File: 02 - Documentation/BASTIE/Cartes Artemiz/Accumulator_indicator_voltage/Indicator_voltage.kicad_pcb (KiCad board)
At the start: 2 copper layers, 82.4 x 42.6 mm, 22 parts, among them J7 2P Droit 2-11-2022, Q1 NMOS SQ2348ES-T1_GE3

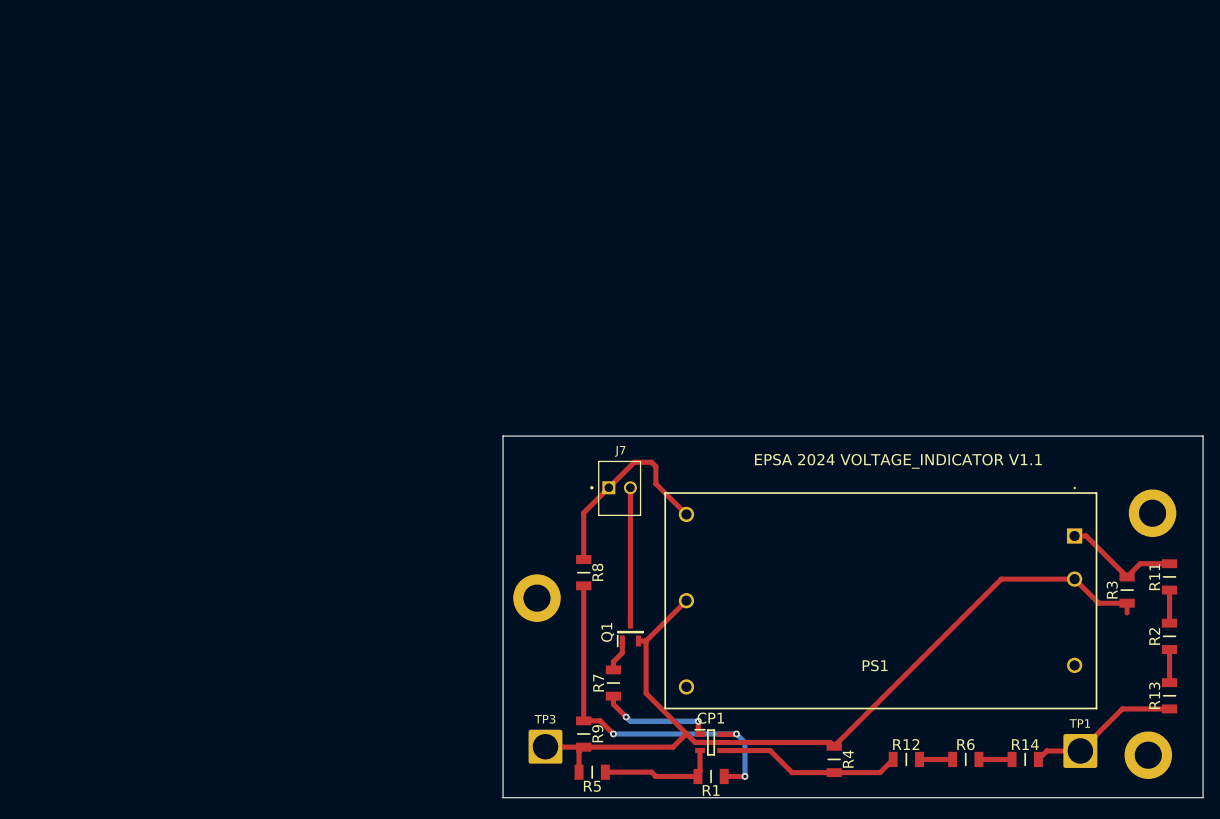
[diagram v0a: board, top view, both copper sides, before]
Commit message: Routage Voltage Indicator
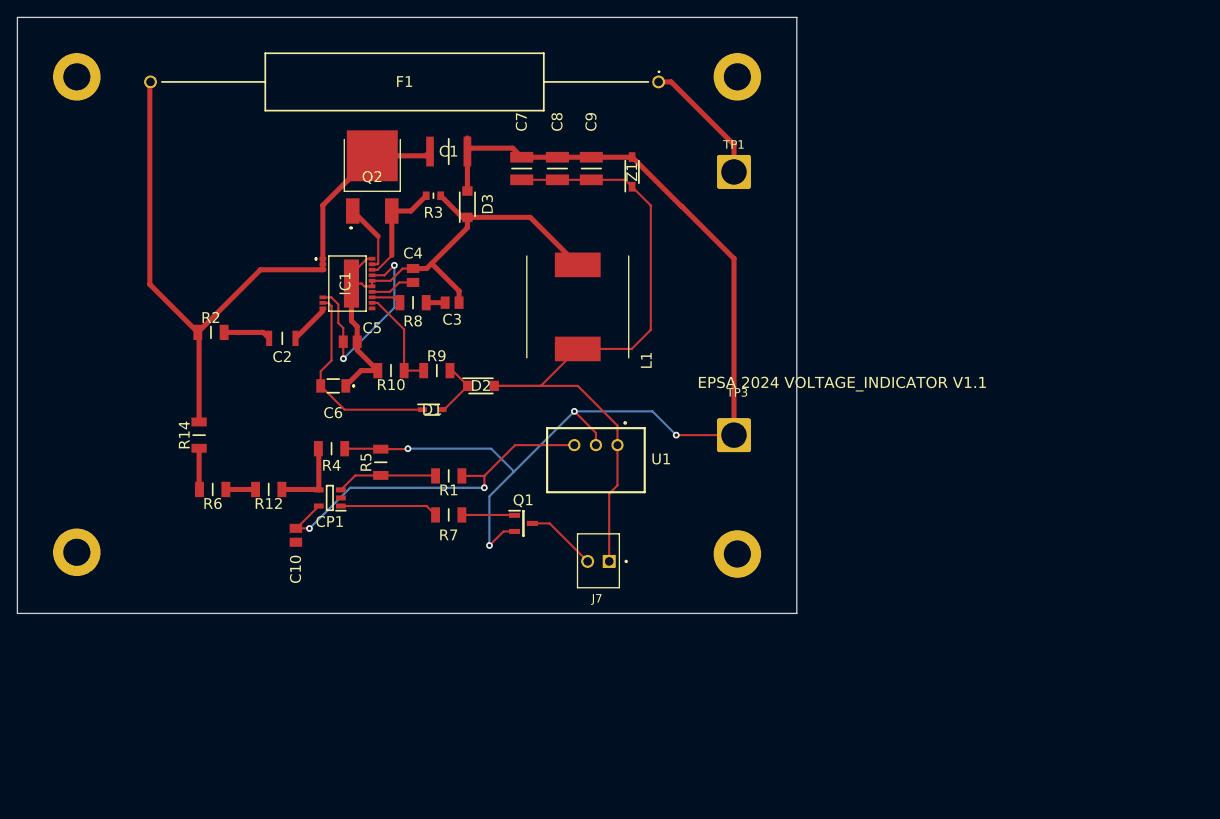
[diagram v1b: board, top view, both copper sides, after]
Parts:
- removed the ? at (93.0, 107.0)
- removed the ? at (165.5, 97.0)
- removed the ? at (165.0, 125.5)
- removed PS1: Alim HP EC7BW18-72S12, EPSA_lib:EC7BW1872S12
- removed R11, R13: 390k, EPSA_lib:RESC3216X70N
- added ?: , , F.Cu at (38.8, 101.6)
- added ?: , , F.Cu at (116.6, 45.6)
- added ?: , , F.Cu at (38.8, 45.6)
- added ?: , , F.Cu at (116.6, 101.8)
- added C1: 0.1u 630V, EPSA_lib:CAPC4532X200N, F.Cu at (82.6, 54.4)
- added C10: 10u, EPSA_lib:CAPC2012X130N, F.Cu at (64.6, 99.6)
- added C2: 10p 630V, EPSA_lib:CAPC3216X100N, F.Cu at (63.0, 76.4)
- added C3: 0.1u, EPSA_lib:CAPC2012X130N, F.Cu at (83.0, 72.2)
- added C4: 0.1u, EPSA_lib:CAPC2012X130N, F.Cu at (78.4, 69.0)
- added C5: 10u, EPSA_lib:CAPC2012X130N, F.Cu at (71.0, 76.8)
- added C6: 10u, EPSA_lib:GRM31x, F.Cu at (69.0, 82.0)
- added C7: 47u, EPSA_lib:CAPC3225X270N, F.Cu at (91.2, 56.4)
- added C8: 47u, EPSA_lib:CAPC3225X270N, F.Cu at (95.4, 56.4)
- added C9: 47u, EPSA_lib:CAPC3225X270N, F.Cu at (99.4, 56.4)
- added D1: Diode CMDSH2-3_TR_PBFREE, EPSA_lib:SOD2512X110N, F.Cu at (80.7, 84.8)
- added D2: Diode US1KFA, EPSA_lib:SODFL3618X143N, F.Cu at (86.4, 82.0)
- added D3: Diode US1KFA, EPSA_lib:SODFL3618X143N, F.Cu at (84.8, 60.6)
- added F1: 200mA, EPSA_lib:0ADAP0200RE, F.Cu at (107.3, 46.2)
- added IC1: Contrôleur LT8316EFE#PBF, EPSA_lib:LT8315EFEPBF, F.Cu at (70.2, 70.0)
- added L1: 1m, EPSA_lib:WE-PD_1260_1245_1280_121054, F.Cu at (97.8, 72.7)
- added Q2: NMOS TK3P80E_RQ, EPSA_lib:TK3P80ERQ, F.Cu at (73.6, 61.4)
- added R10: 2.4k, EPSA_lib:RESC3216X70N, F.Cu at (75.8, 80.2)
- added U1: Alim LP TSR_0.5-2450, EPSA_lib:TSR-0.5-2433, F.Cu at (105.7, 87.0)
- added Z1: Diode Zener CMHZ4107_TR_PBFREE, EPSA_lib:SOD3816X135N, F.Cu at (104.2, 56.8)
- R2: value 390k -> 10k
- R3: value 390k -> 0.22; footprint EPSA_lib:RESC3216X70N -> EPSA_lib:RESC1608X55N
- R8: value 5k6 -> 22k
- R9: value 3k9 -> 22k
- moved R2 118.4 mm to (54.6, 75.7), turned to 0 degrees
- moved R14 104.5 mm to (53.2, 87.8), turned to 90 degrees
- moved R6 94.2 mm to (54.8, 94.2), turned to 180 degrees
- moved R3 94.0 mm to (80.8, 59.6), turned to 0 degrees
- moved R12 81.6 mm to (61.4, 94.2), turned to 180 degrees
- moved TP1 79.5 mm to (116.2, 56.8)
- moved R4 69.6 mm to (68.8, 89.4), turned to 180 degrees
- moved CP1 53.3 mm to (68.6, 95.2), turned to 180 degrees
- moved R1 47.0 mm to (82.6, 92.6)
- moved R9 46.2 mm to (81.2, 80.2), turned to 0 degrees
- moved R5 44.2 mm to (74.6, 91.0), turned to 90 degrees
- moved TP3 42.9 mm to (116.2, 87.8)
- moved R8 37.6 mm to (78.4, 72.2), turned to 0 degrees
- moved R7 27.7 mm to (82.6, 97.2), turned to 0 degrees
- moved Q1 18.0 mm to (91.4, 98.2), turned to 0 degrees
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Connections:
- CP1 pad 5: 5V -> +5V
- J7 pad 1: 12V -> +12V
- R1 pad 1: 5V -> +5V
- R2 pad 1: Net-(R13-Pad2) -> HV+
- R3 pad 1: 0 -> Net-(IC1-SENSE)
- R3 pad 2: /150V -> Net-(D3-K)
- R8 pad 1: 12V -> Net-(IC1-VC)
- R8 pad 2: 5V -> Net-(C3-Pad1)
- R9 pad 1: 5V -> Net-(IC1-FB)
- R9 pad 2: 0 -> Net-(D1-A)
- TP1 pad 1: HV+ -> HV in
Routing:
- net +12V: track 0.00 -> 85.2 mm
- net HV+: track 17.9 -> 83.1 mm
- net Net-(D3-K): track 0.00 -> 64.1 mm
- net +5V: track 0.00 -> 44.1 mm, vias 0 -> 2
- net 5V: track 44.1 -> 0.00 mm, vias 3 -> 0
- net 0: track 103.9 -> 133.8 mm, vias 0 -> 4
- net Net-(IC1-EN/UVLO): track 0.00 -> 25.4 mm, vias 0 -> 2
- net Net-(D1-K): track 0.00 -> 24.2 mm
- net 12V: track 23.8 -> 0.00 mm
- net HV in: track 0.00 -> 15.1 mm
- net /150V: track 13.8 -> 0.00 mm
- net Net-(IC1-SENSE): track 0.00 -> 13.1 mm
- net Net-(CP1-IN+): track 21.9 -> 9.24 mm
- net Net-(IC1-FB): track 0.00 -> 12.2 mm
- net Net-(IC1-GATE): track 0.00 -> 8.20 mm
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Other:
- board size 82.4 x 42.6 mm -> 91.8 x 70.2 mm
